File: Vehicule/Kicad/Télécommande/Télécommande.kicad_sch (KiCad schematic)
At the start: 5 parts, among them J1 Conn_01x02_Socket, U1 ESP32-C3_SUPERMINI

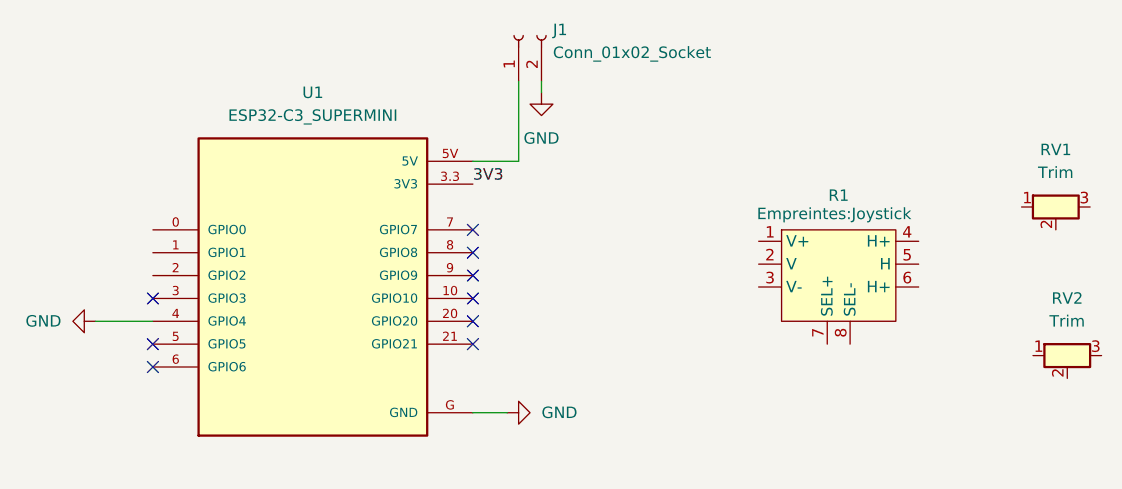
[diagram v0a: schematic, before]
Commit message: Compléter le schéma
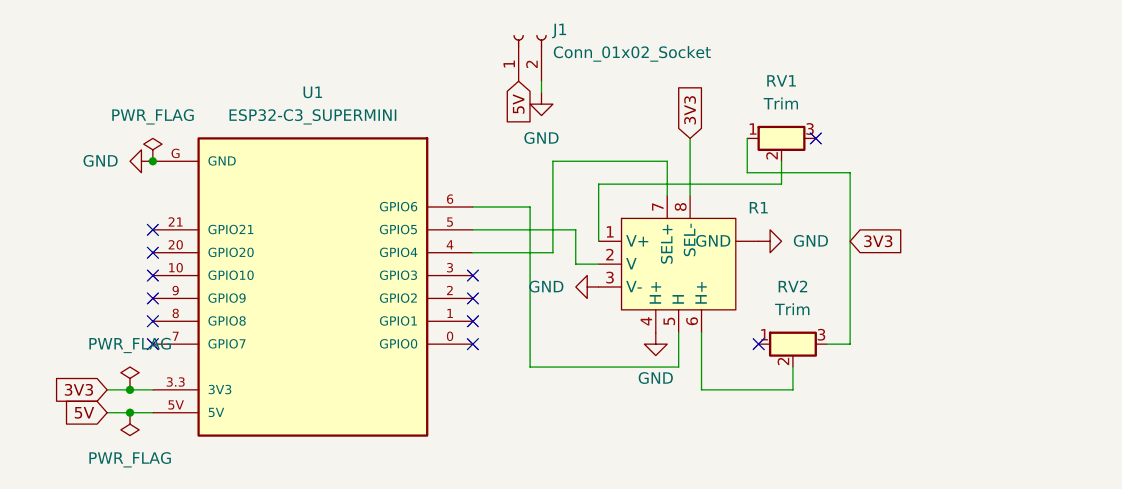
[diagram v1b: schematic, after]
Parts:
- R1: footprint Empreintes:Joystick -> (none)
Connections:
- net 3V3: now also R1.8 (SEL-), RV1.1, RV2.3
- net GND: now also R1. (GND), R1.3 (V-), R1.4 (H+); no longer U1.4 (GPIO4)
- net at RV1.2: now also R1.1 (V+)
- net at RV2.2: now also R1.6 (H+)
- net at R1.2 (V): now also U1.5 (GPIO5)
- net at R1.5 (H): now also U1.6 (GPIO6)
- net at R1.7 (SEL+): now also U1.4 (GPIO4)
- net 5V: now reaches J1.1 (Pin_1), U1.5V
- no-connect marks 9 -> 12
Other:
- moved on the sheet: RV1, RV2, U1
